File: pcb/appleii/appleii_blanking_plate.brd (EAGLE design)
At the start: 75 x 45 mm, 21 parts, among them J1 ATX24RH

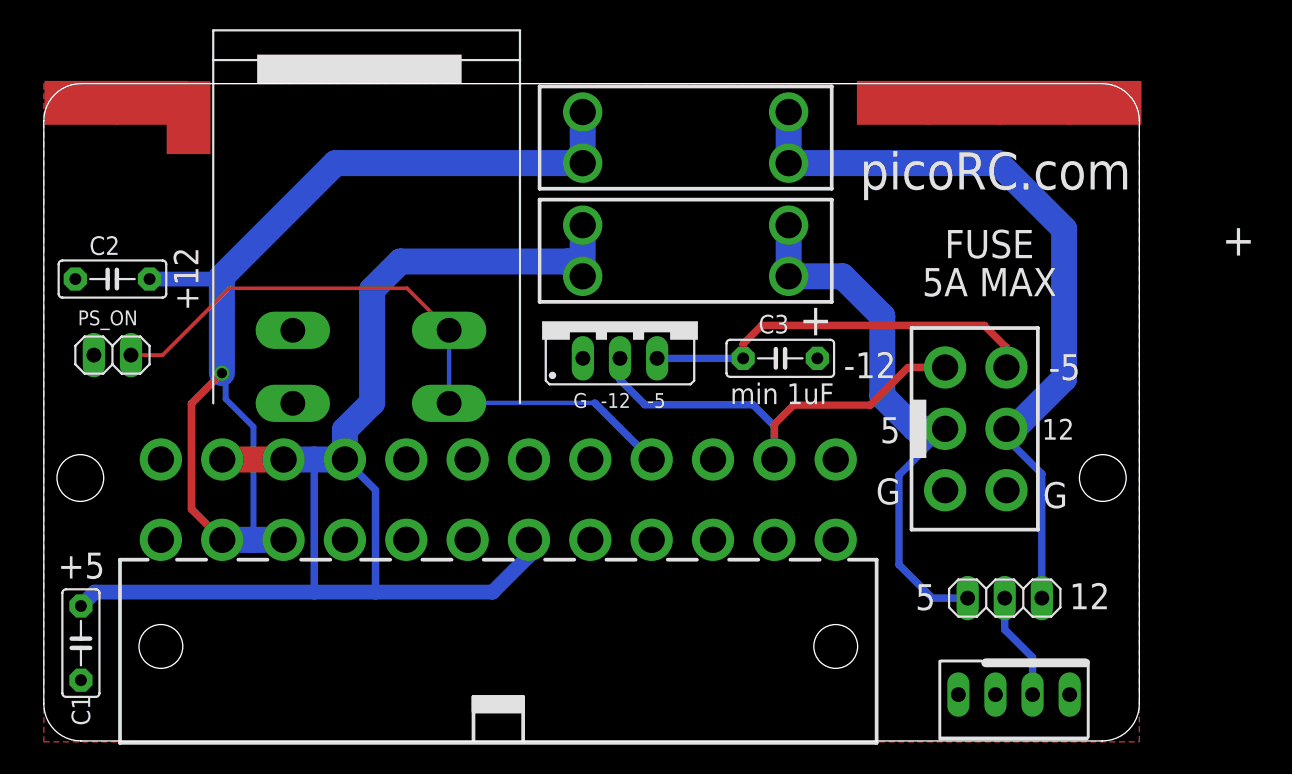
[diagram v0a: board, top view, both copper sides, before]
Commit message: updated IIGS design
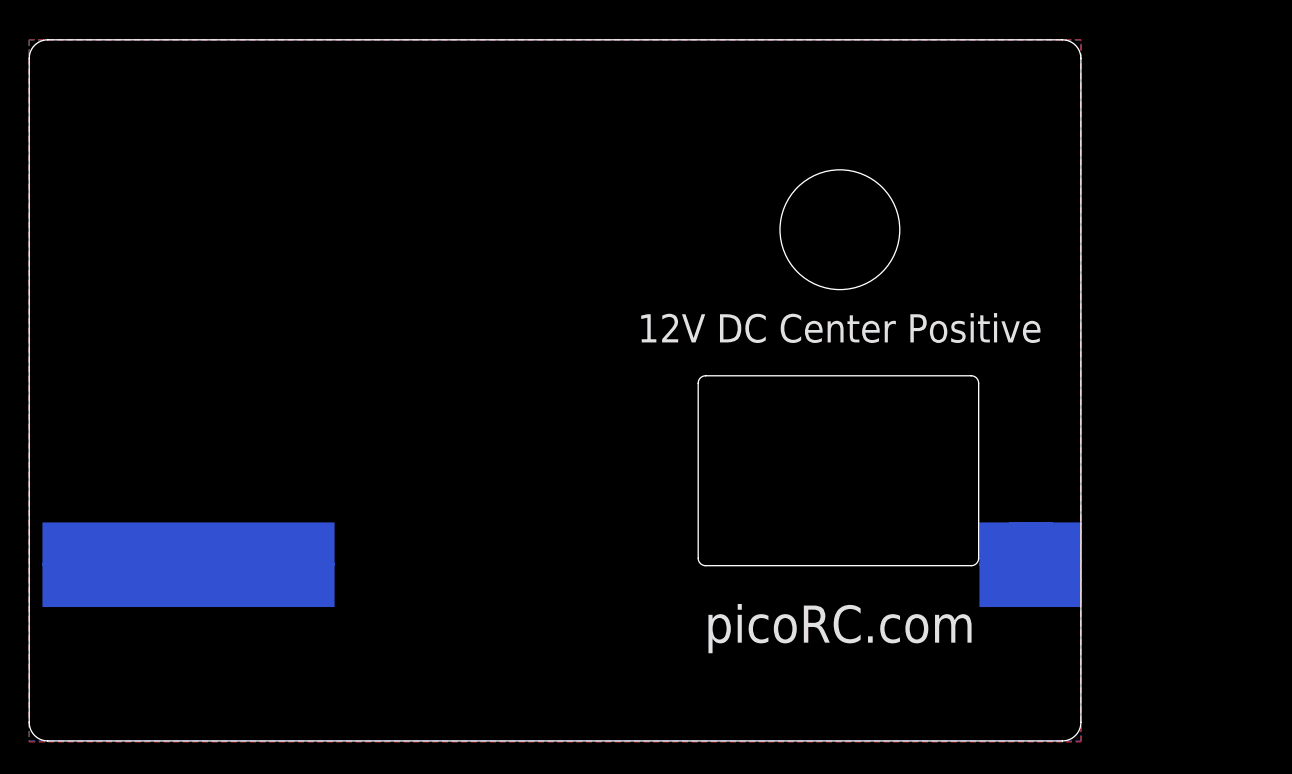
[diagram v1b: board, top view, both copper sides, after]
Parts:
- removed C1, C2, C3: (no value), capacitor-wima:C5B2.5
- removed IC1: (no value), v-reg:79XXS
- removed J1: ATX24RH, macse:ATX24_RIGHT_ANGLE
- removed JP1: (no value), pinhead:1X02
- removed JP2: (no value), pinhead:1X03
- removed JP3: (no value), appleii:1X04
- removed U$10, U$11, U$12, U$7, U$8, U$9: EDGEPAD, atx4vc:EDGEPAD
- removed U$6: APPLEII, atx4vc:APPLEII
- U$1: value CAR_FUSE_HOLDER3IN1 -> EDGEPADEDGEPAD_20MM; device atx_power_control:FUSE_HOLDER_3IN1 -> atx4vc:EDGEPAD_20MM
- U$2: value CAR_FUSE_HOLDER3IN1 -> EDGEPAD; device atx_power_control:FUSE_HOLDER_3IN1 -> atx4vc:EDGEPAD
- U$3: value ROCK_SW -> EDGEPAD; device atx4vc:ROCK_SWITCH -> atx4vc:EDGEPAD
- U$4: value M3_MOUNTING_HOLE -> EDGEPAD; device a:M3_MOUNTING_HOLE_PACK -> atx4vc:EDGEPAD
- U$5: value M3_MOUNTING_HOLE -> EDGEPADEDGEPAD_20MM; device a:M3_MOUNTING_HOLE_PACK -> atx4vc:EDGEPAD_20MM
- moved U$3 48.1 mm to (68.6, 10.7), flipped to the bottom, turned to 270 degrees
- moved U$1 39.5 mm to (9.91, 13.5), flipped to the bottom, turned to 270 degrees
- moved U$2 35.9 mm to (66.5, 13.5), flipped to the bottom, turned to 270 degrees
- moved U$13 30.5 mm to (68.6, 13.5), flipped to the bottom
- moved U$5 10.4 mm to (9.91, 10.7), flipped to the bottom, turned to 270 degrees
- moved U$4 9.44 mm to (66.5, 10.7), flipped to the bottom, turned to 270 degrees
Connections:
- removed net +12V: JP2.3, U$2.B0, U$2.B1, U$6.4
- removed net +5V: JP2.1, U$1.A0, U$1.A1, U$6.3
- removed net -12V: IC1.IN, J1.14, U$6.5
- removed net -5V: C3.1, IC1.OUT, U$6.6
- removed net N$1: JP2.2, JP3.2
- removed net N$5: J1.16, JP1.1, U$3.P$2, U$3.P$4
- removed net N$6: C1.1, J1.21, J1.22, J1.23, J1.6, U$1.B0, U$1.B1
- removed net N$8: C2.1, J1.10, J1.11, U$2.A0, U$2.A1
- net GND: now also U$1.P$1, U$2.P$1, U$4.P$1, U$5.P$1; no longer C1.2, C2.2, C3.2, IC1.GND, J1.15, J1.17, J1.18, J1.19, J1.24, J1.3, J1.5, J1.7, JP1.2, JP3.1, U$10.P$1, U$11.P$1, U$12.P$1, U$3.P$3, U$6.1, U$6.2, U$7.P$1, U$8.P$1, U$9.P$1
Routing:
- net N$6: track 92.1 -> 0.00 mm
- net N$8: track 85.8 -> 0.00 mm, vias 1 -> 0
- net +12V: track 52.4 -> 0.00 mm
- net N$5: track 45.3 -> 0.00 mm
- net +5V: track 38.0 -> 0.00 mm
- net -12V: track 31.4 -> 0.00 mm
- net -5V: track 27.4 -> 0.00 mm
- net N$1: track 7.39 -> 0.00 mm
- added copper zone on layer 16, net GND
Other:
- board size 75 x 45 mm -> 72 x 48 mm
- board text added: "12V DC Center Positive"
- board text removed: "+"
- board text removed: "+12"
- board text removed: "+5"
- board text removed: "-12"
- board text removed: "-5"
- board text removed: "12"
- board text removed: "5"
- board text removed: "Apple II / II Plus / IIe PicoPSU Adaptor"
- board text removed: "FUSE 5A MAX"
- board text removed: "G"
- board text removed: "Instructions: picoRC.com"
- board text removed: "PD2 dekuNukem APR23"
- board text removed: "PS_ON"
- board text removed: "min 1uF"
